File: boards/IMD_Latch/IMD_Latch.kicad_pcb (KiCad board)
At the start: 2 copper layers, 32 parts, among them J1 micromatch_female_RA_8, J2 Ultrafit_2, K1 G5Q-1A4-DC5-5V, Q1 SSM3K333R, U1 TPS561201, U2 TLP175A_OEM, U3 TS507IYLT

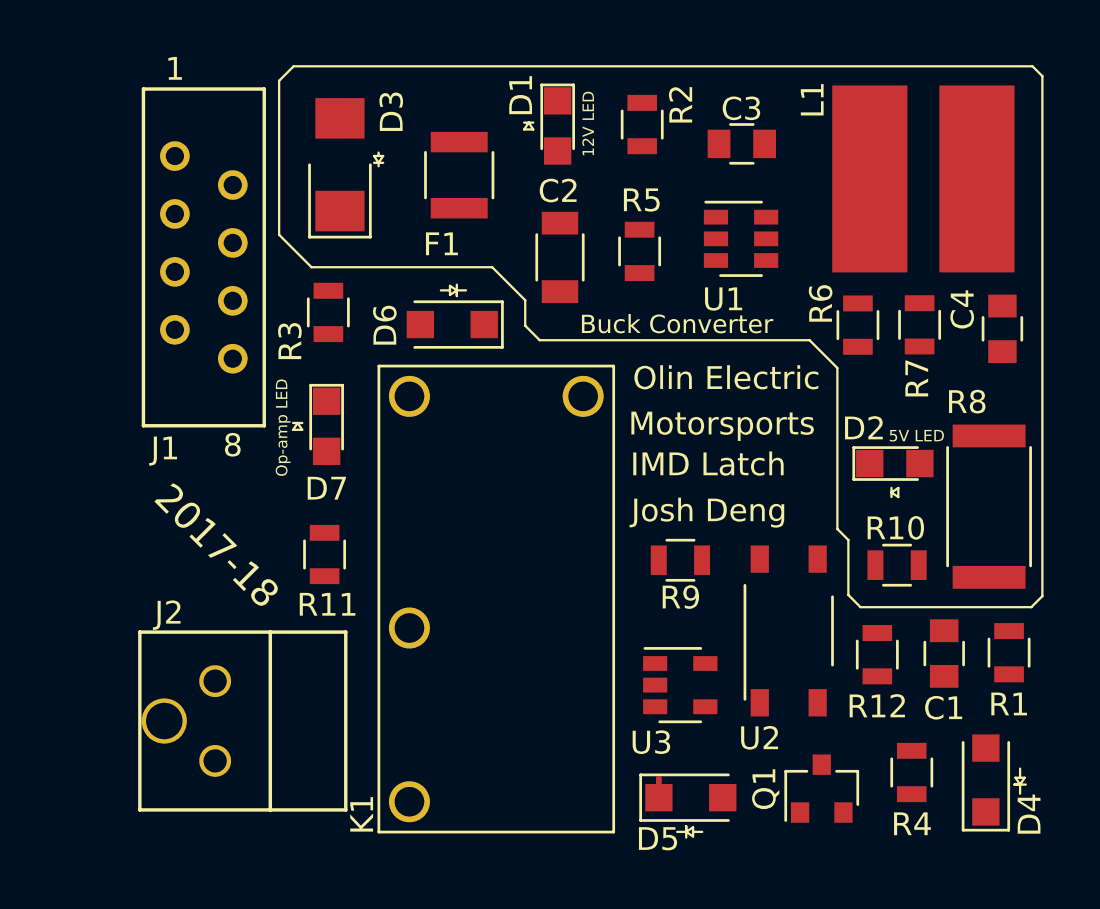
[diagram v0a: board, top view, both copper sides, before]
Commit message: Layout finished
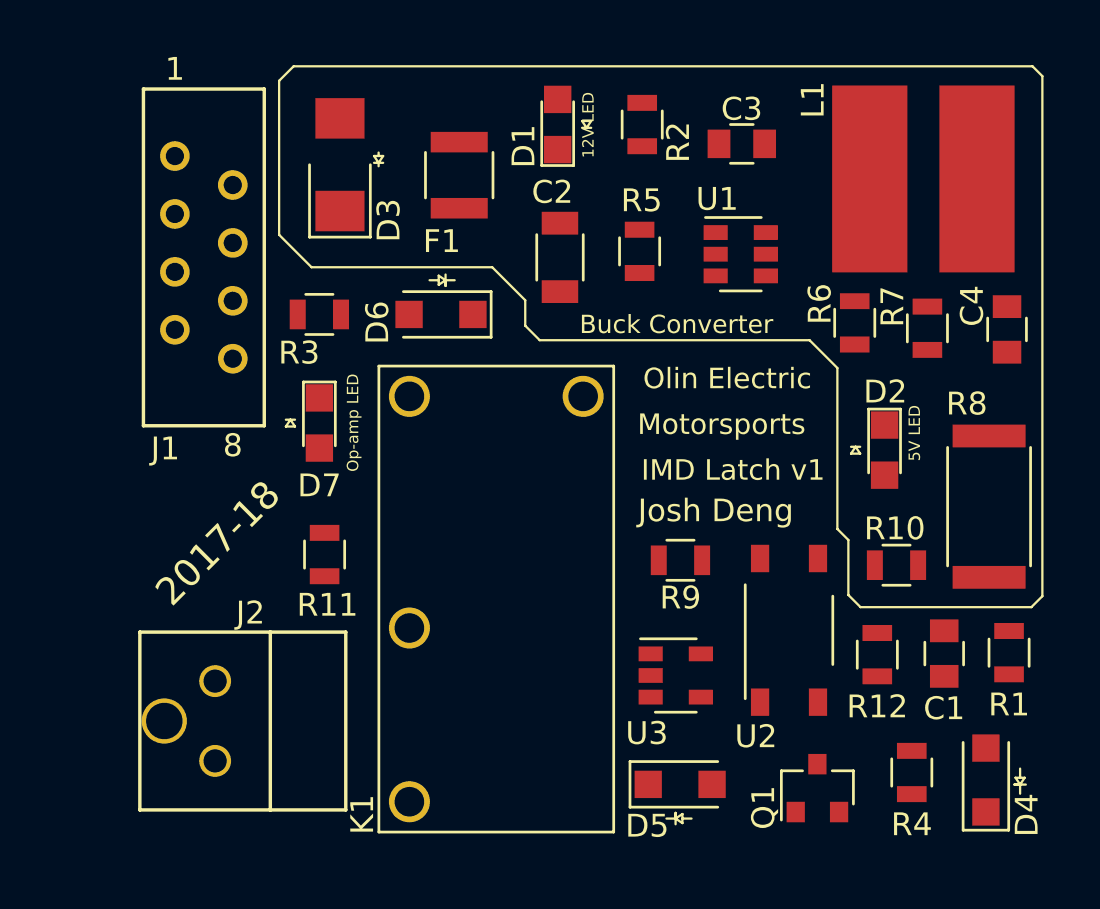
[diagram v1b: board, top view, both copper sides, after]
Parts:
- moved D5 0.75 mm to (154.4, 118.8)
- moved D2 0.74 mm to (163.4, 104.1), turned to 270 degrees
- moved U1 0.67 mm to (157.1, 95.5)
- moved D6 0.67 mm to (143.9, 98.2)
- moved U3 0.46 mm to (154.2, 114.0)
- moved R3 0.40 mm to (138.6, 98.2), turned to 0 degrees
- moved R7 0.37 mm to (165.2, 98.8)
- moved D7 0.35 mm to (138.6, 102.9)
- moved C4 0.20 mm to (168.7, 98.8), turned to 270 degrees
- moved Q1 0.19 mm to (160.4, 119.0)
- moved R6 0.17 mm to (162.1, 98.6), turned to 270 degrees
- moved D1 0.06 mm to (149.0, 89.9), turned to 90 degrees
- turned R2 to 90 degrees
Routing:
- net Net-(D5-Pad1): track 0.85 -> 0.00 mm
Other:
- board text added: "IMD Latch v1"
- board text removed: "IMD Latch"

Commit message: Tracing ready Layout
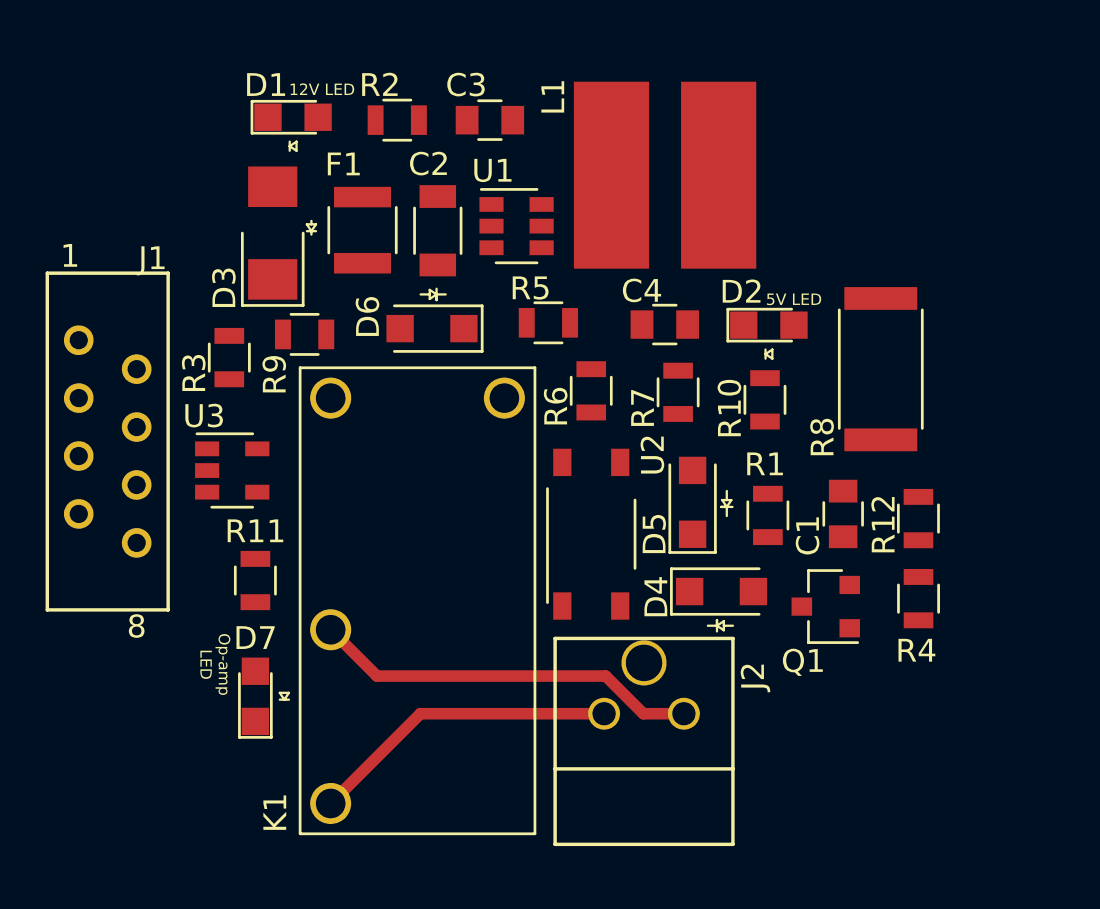
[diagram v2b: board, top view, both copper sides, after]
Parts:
- moved U3 21.4 mm to (134.7, 105.0)
- moved R9 19.2 mm to (137.9, 99.1)
- moved J2 17.2 mm to (151.1, 115.7), turned to 90 degrees
- moved C4 15.0 mm to (153.7, 98.6), turned to 180 degrees
- moved D4 14.2 mm to (156.2, 110.3), turned to 0 degrees
- moved D5 12.4 mm to (154.9, 106.4), turned to 90 degrees
- moved D7 12.3 mm to (135.8, 114.9), turned to 90 degrees
- moved R1 12.2 mm to (158.2, 107.0)
- moved R6 11.9 mm to (150.5, 101.5), turned to 90 degrees
- moved D1 11.6 mm to (137.4, 89.5), turned to 0 degrees
- moved L1 11.3 mm to (153.7, 92.1)
- moved R7 11.3 mm to (154.3, 101.6)
- moved C3 11.1 mm to (146.1, 89.7)
- moved R2 10.7 mm to (142.0, 89.7), turned to 180 degrees
- moved U1 9.91 mm to (147.2, 94.3)
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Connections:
- D5 pad 1: Net-(D5-Pad1) -> Net-(D4-Pad1)
- D5 pad 2: Net-(D4-Pad1) -> Net-(D5-Pad2)
- D6 pad 1: Net-(D5-Pad1) -> Net-(D5-Pad2)
- K1 pad 5: Net-(D5-Pad1) -> Net-(D5-Pad2)
- U2 pad 4: Net-(D5-Pad1) -> Net-(D5-Pad2)
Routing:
- net Net-(J2-Pad1): track 0.00 -> 17.0 mm
- net Net-(J2-Pad2): track 0.00 -> 13.6 mm
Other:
- board text removed: "Buck Converter"
- board text removed: "Motorsports"
- board text removed: "Olin Electric"

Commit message: IMD Latch Tracing for the first time
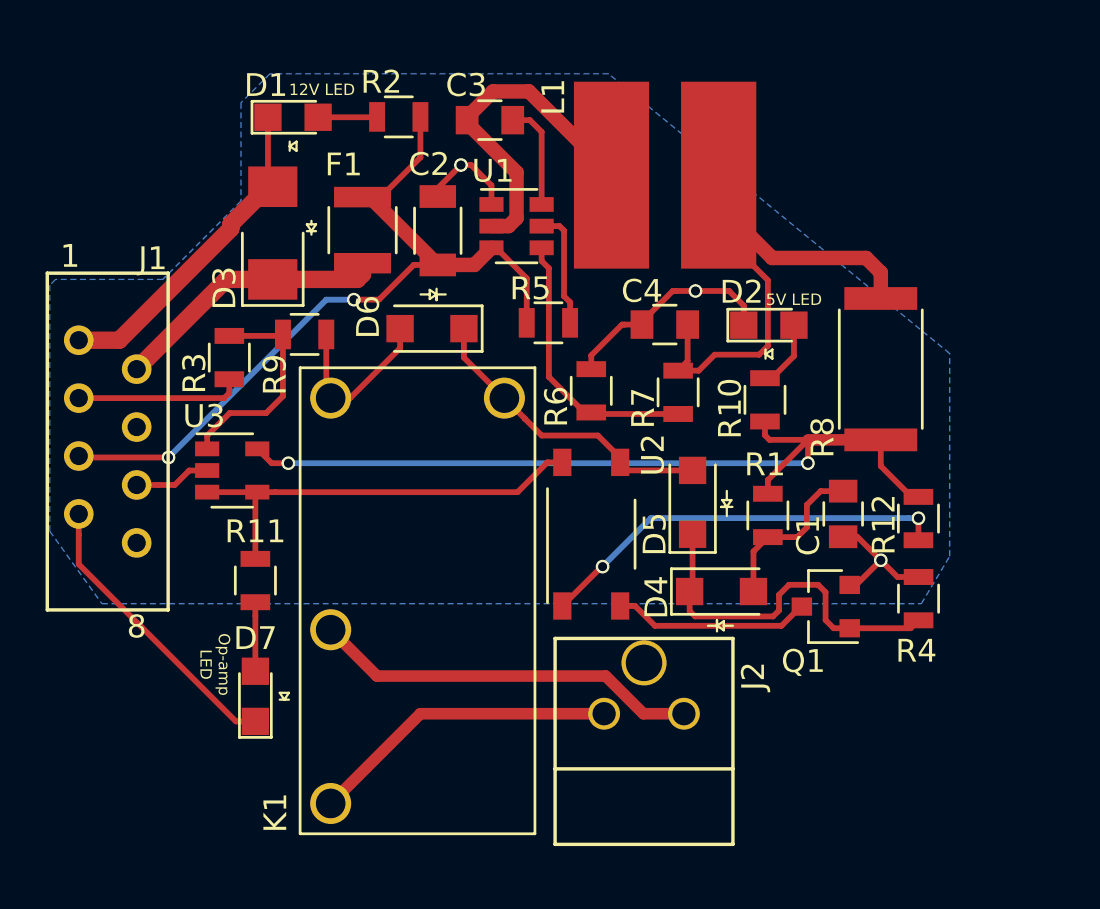
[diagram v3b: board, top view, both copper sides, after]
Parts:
- moved R2 0.16 mm to (142.1, 89.5)
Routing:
- net GND: track 0.00 -> 58.2 mm, vias 0 -> 3
- net VCC: track 0.00 -> 40.9 mm, vias 0 -> 2
- net /12V_Fused: track 0.00 -> 35.6 mm, vias 0 -> 2
- net Net-(C4-Pad1): track 0.00 -> 25.7 mm
- net Net-(R11-Pad1): track 0.00 -> 19.1 mm
- net Net-(R12-Pad1): track 0.00 -> 18.2 mm, vias 0 -> 2
- net Net-(D4-Pad1): track 0.11 -> 16.3 mm
- net Net-(C3-Pad2): track 0.00 -> 14.9 mm
- net Net-(D5-Pad2): track 0.00 -> 13.5 mm
- net Net-(R6-Pad1): track 0.00 -> 12.1 mm
- net +12V: track 0.00 -> 12.1 mm
- net Net-(R3-Pad2): track 0.00 -> 9.71 mm
- net Net-(Q1-Pad3): track 0.00 -> 8.68 mm
- net Net-(C1-Pad1): track 0.12 -> 7.49 mm
- net Net-(J1-Pad3): track 0.00 -> 7.30 mm
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- added copper zone on B.Cu, net GND
